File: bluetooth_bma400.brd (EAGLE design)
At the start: 38.1 x 38.1 mm, 20 parts, among them IC1 BLUENRG-M2SP, J2 455-1750-1-ND, U1 BMA400

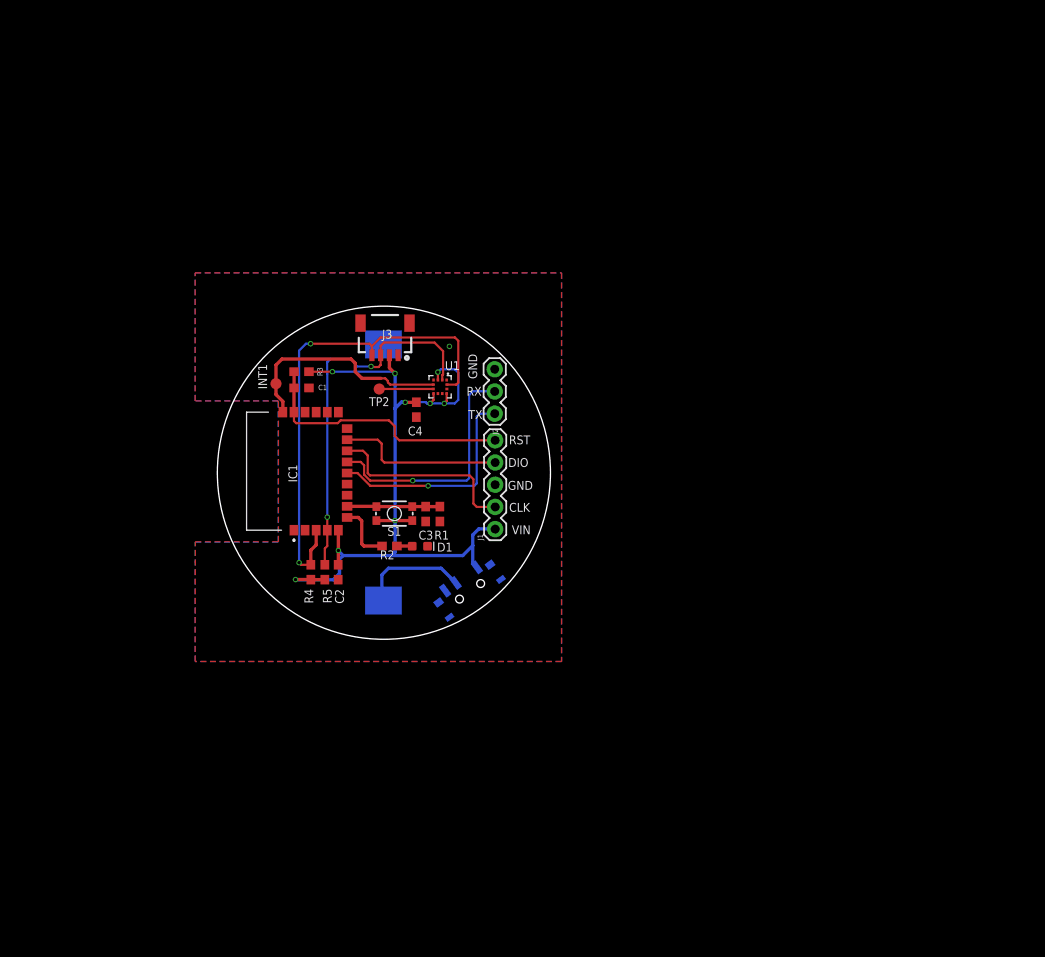
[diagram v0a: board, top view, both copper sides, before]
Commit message: Updated files
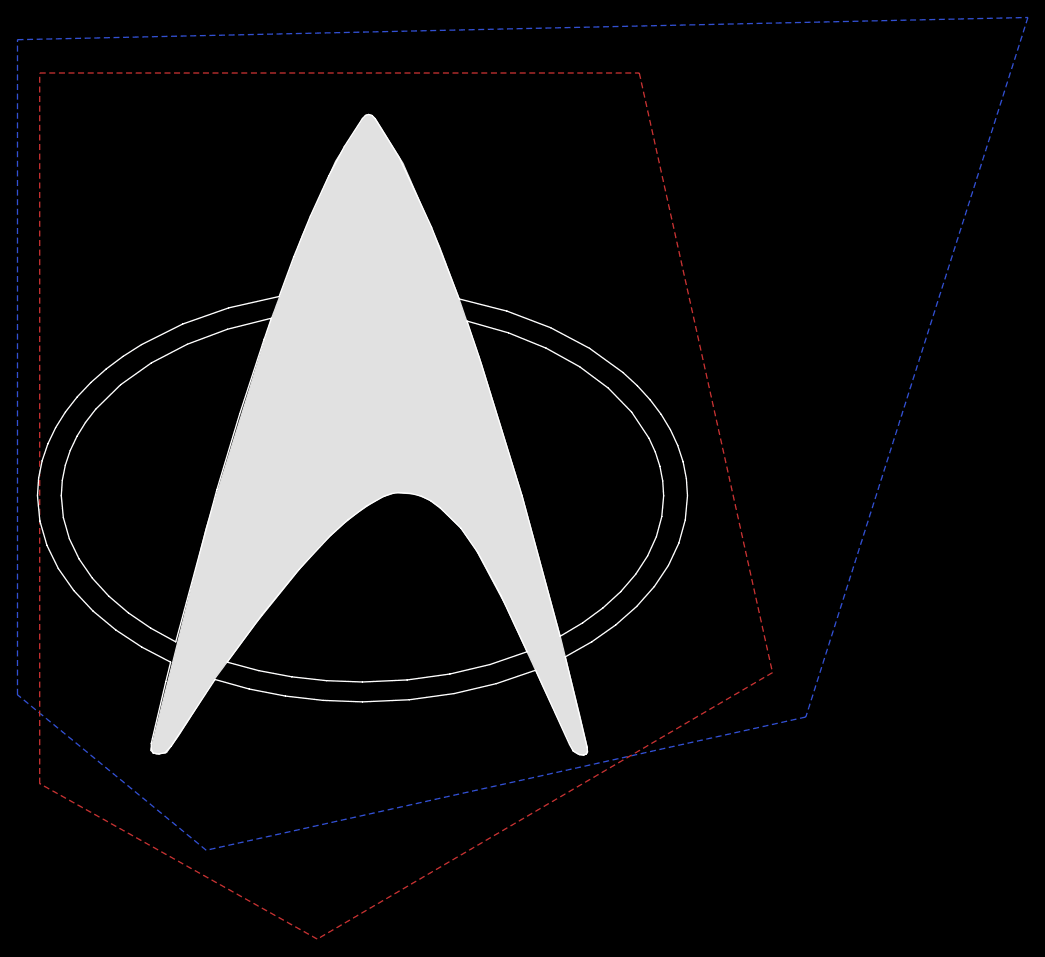
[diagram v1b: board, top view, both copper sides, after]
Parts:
- removed BT1: BU2032SM-JJ-GTR, BU2032SM-JJ-GTR:BAT_BU2032SM-JJ-GTR
- removed C4: 10nF, SparkFun-Capacitors:0603
- removed INT1, TP2: TPB1,27, testpad:B1,27
- removed R4, R5: 2.2k, SparkFun-Resistors:0603
- removed S2: (no value), SparkFun-Switches:SWITCH_SPST_SMD_A
- removed U1: BMA400, BMA400:XDCR_BMA400
- moved J1 28.7 mm to (-15.3, 0.10), turned to 270 degrees
- moved J2 25.6 mm to (-10.2, -4.67)
- moved C2 20.7 mm to (8.74, 3.86)
- moved IC1 16.0 mm to (-1.09, 14.1), turned to 0 degrees
- moved R3 13.7 mm to (-1.80, 23.0)
- moved J3 12.8 mm to (-1.14, 26.1)
- moved R2 12.0 mm to (6.99, 1.78)
- moved C3 10.2 mm to (4.78, 5.44)
- moved D1 9.25 mm to (13.0, -5.87)
- moved S1 6.84 mm to (-1.35, 1.68)
- moved C1 6.35 mm to (-9.42, 3.35)
- moved R1 6.35 mm to (11.5, -0.91)
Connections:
- removed net INT2: TP2.TP, U1.6
- removed net N$2: BT1.+, S2.2
- net GND: no longer BT1.-, C4.1, U1.1, U1.8, U1.9
- net INT1: no longer INT1.TP, U1.5
- net SCL: no longer R4.1, U1.12
- net SDA: no longer R5.1, U1.2
- net VIN: no longer C4.2, R4.2, R5.2, S2.3, U1.10, U1.3, U1.7
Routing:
- net VIN: track 93.4 -> 0.00 mm, vias 9 -> 0
- net SCL: track 56.4 -> 0.00 mm, vias 2 -> 0
- net SDA: track 43.4 -> 0.00 mm, vias 2 -> 0
- net RST: track 30.5 -> 0.00 mm
- net RX: track 28.2 -> 0.00 mm, vias 1 -> 0
- net INT1: track 25.9 -> 0.00 mm
- net TX: track 25.4 -> 0.00 mm, vias 1 -> 0
- net SWCLK: track 22.4 -> 0.00 mm
- net SWDIO: track 19.1 -> 0.00 mm
- net N$2: track 12.5 -> 0.00 mm
- net BOOT: track 10.6 -> 0.00 mm
- net TEST: track 6.88 -> 0.00 mm
- net INT2: track 6.19 -> 0.00 mm
- net N$1: track 1.76 -> 0.00 mm
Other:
- board size 38.1 x 38.1 mm -> 74.3 x 73.2 mm
- board text removed: "03-01-2021"
- board text removed: "CLK"
- board text removed: "DIO"
- board text removed: "GND"
- board text removed: "Low Cost Pedometer"
- board text removed: "RST"
- board text removed: "RX"
- board text removed: "TX"
- board text removed: "VIN"
